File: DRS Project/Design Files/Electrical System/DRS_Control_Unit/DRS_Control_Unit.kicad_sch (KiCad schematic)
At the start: 32 parts, among them J1 Deutsch DT, J2 Servo, J3 Screw, U1 AMS1117, U2 LM2596S-ADJ, U3 Teensy4.0-NU-Teams, U4 TJA1051T-3

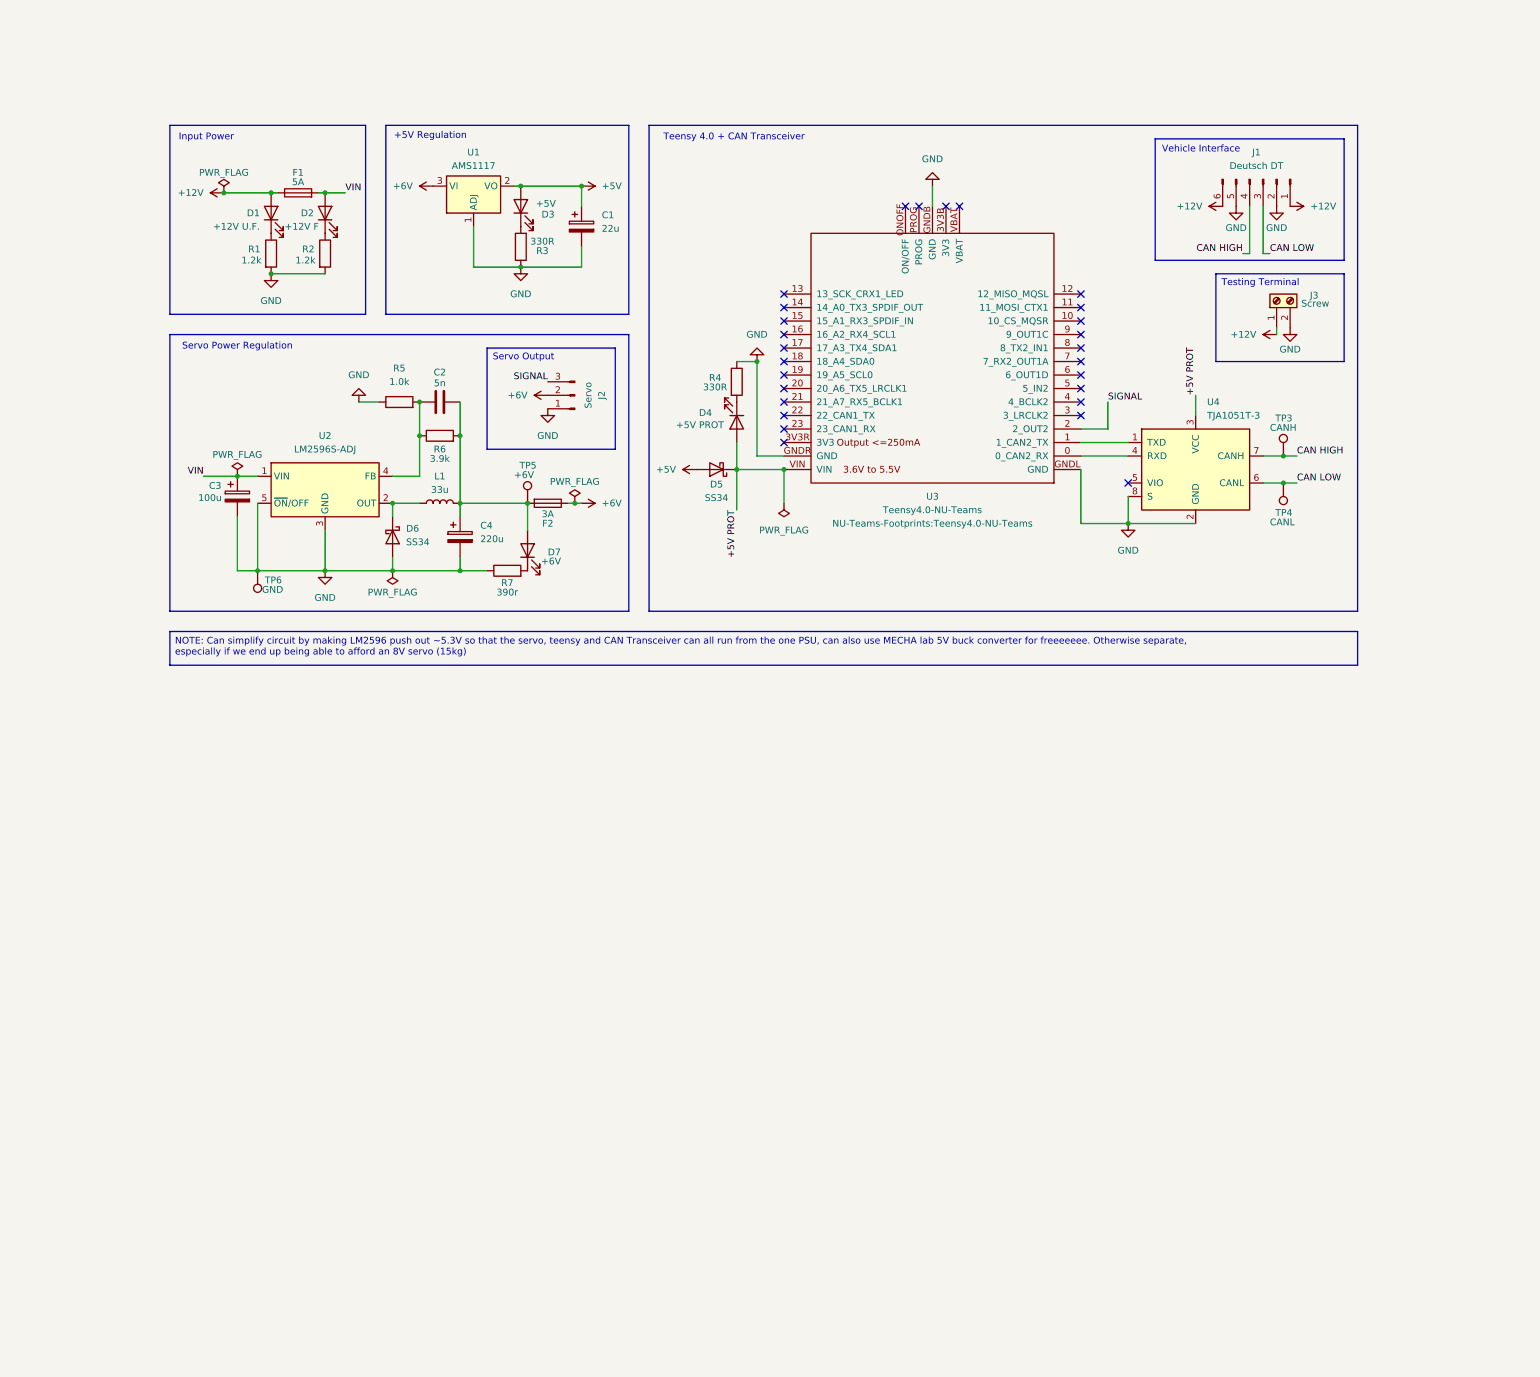
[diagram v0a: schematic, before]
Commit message: nearly finised circuit v1.1
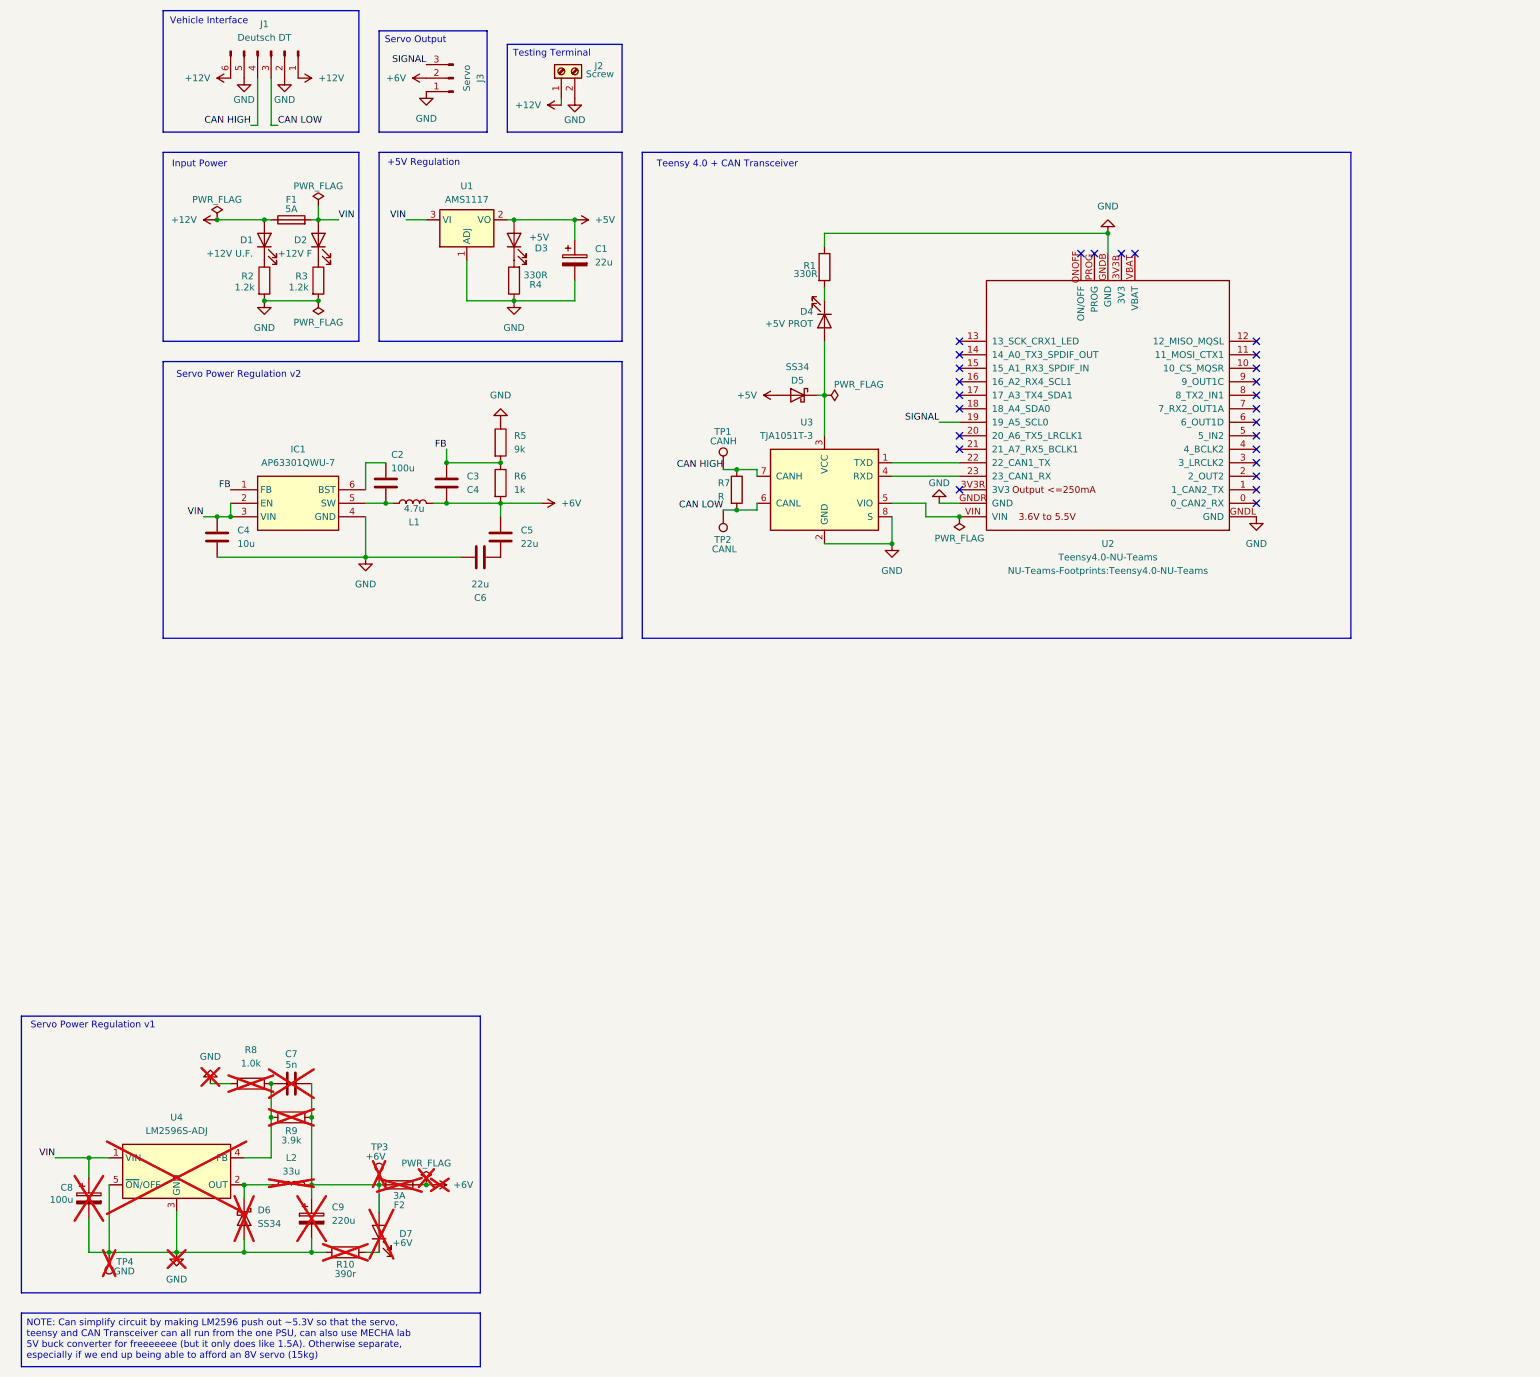
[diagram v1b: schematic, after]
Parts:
- added C2: 100u, Capacitor_SMD:C_1206_3216Metric_Pad1.33x1.80mm_HandSolder, symbol Device:C
- added C3: C4, Capacitor_SMD:C_1206_3216Metric_Pad1.33x1.80mm_HandSolder, symbol Device:C
- added C4: 10u, Capacitor_SMD:C_1206_3216Metric_Pad1.33x1.80mm_HandSolder, symbol Device:C
- added C5, C6: 22u, Capacitor_SMD:C_1206_3216Metric_Pad1.33x1.80mm_HandSolder, symbol Device:C
- added IC1: AP63301QWU-7, DRS_Library:TSOT-26, symbol AP63301QWU-7:AP63301QWU-7
- added L1: 4.7u, symbol Device:L
- added R5: 9k, Resistor_SMD:R_1206_3216Metric_Pad1.30x1.75mm_HandSolder, symbol Device:R
- added R6: 1k, Resistor_SMD:R_1206_3216Metric_Pad1.30x1.75mm_HandSolder, symbol Device:R
- added R7: R, Resistor_SMD:R_1206_3216Metric_Pad1.30x1.75mm_HandSolder, symbol Device:R
- C7: renamed from C2; now not fitted
- C8: renamed from C3; now not fitted
- C9: renamed from C4; now not fitted
- D6, D7, F2: now not fitted
- J3: renamed from J2; footprint Connector_PinHeader_2.54mm:PinHeader_1x03_P2.54mm_Vertical -> Connector_PinHeader_2.54mm:PinHeader_1x03_P2.54mm_Horizontal
- L2: renamed from L1; now not fitted
- R10: renamed from R7; now not fitted
- R8: renamed from R5; now not fitted
- R9: renamed from R6; now not fitted
- TP3: renamed from TP5; now not fitted
- TP4: renamed from TP6; now not fitted
- U4: renamed from U2; now not fitted
- renumbered J3 to J2, R4 to R1, R1 to R2, R2 to R3, R3 to R4, TP3 to TP1, TP4 to TP2, U3 to U2, U4 to U3
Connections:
- net +6V: now also C3.2, C5.1, L1.2, R6.2; no longer U1.3 (VI)
- net CAN HIGH: now also R7.1
- net CAN LOW: now also R7.2
- net GND: now also C4.2, C6.2, IC1.4 (GND), R5.1
- net SIGNAL: now also U2.19 (19_A5_SCL0); no longer U2.2 (2_OUT2)
- net VIN: now also U1.3 (VI), C4.1, IC1.2 (EN), IC1.3 (VIN)
- net at U2.0 (0_CAN2_RX): no longer U3.4 (RXD)
- net at U2.1 (1_CAN2_TX): no longer U3.1 (TXD)
- net at U2.22 (22_CAN1_TX): now also U3.1 (TXD)
- net at U2.23 (23_CAN1_RX): now also U3.4 (RXD)
- net at U3.5 (VIO): now also U2.VIN
- net +5V PROT: no longer names the net of D4.2 (A), D5.1 (K), U3.3 (VCC)
- net +5V PROT: no longer U2.VIN
- new net: C2.2, IC1.5 (SW), L1.1
- new net: C2.1, IC1.6 (BST)
- new net: C5.2, C6.1
- new net FB: C3.1, IC1.1 (FB), R5.2, R6.1
- no-connect marks 27 -> 26
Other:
- note added: "Servo Power Regulation v1"
- note added: "Servo Power Regulation v2"
- note removed: "Servo Power Regulation"
- moved on the sheet: C1, D1, D2, D3, D4, D5, F1, J1, J2, J3, R1, R2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
